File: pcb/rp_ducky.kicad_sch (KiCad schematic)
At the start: 31 parts, among them J1 USB_A, SW1 R-667799, SW2 R-667799, U1 TCR2EE33, U2 W25Q32JVZP, U3 RP2040, Y1 Crystal_GND24

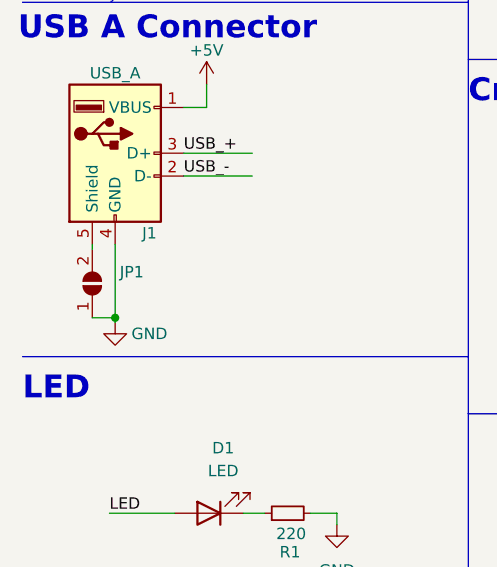
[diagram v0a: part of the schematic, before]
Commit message: WIP
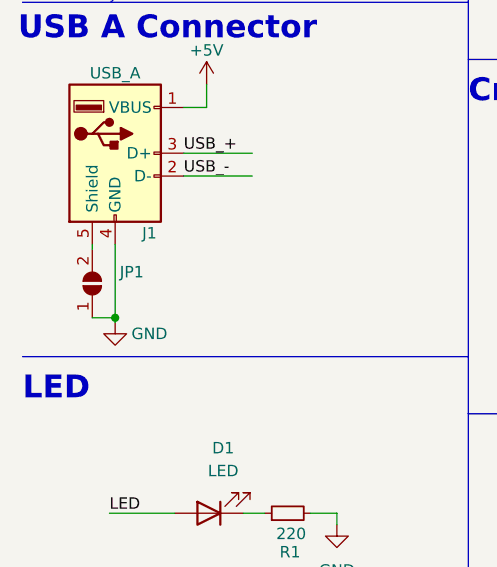
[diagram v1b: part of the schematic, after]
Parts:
- JP1: footprint Jumper:SolderJumper-2_P1.3mm_Open_TrianglePad1.0x1.5mm -> Jumper:SolderJumper-2_P1.3mm_Bridged_RoundedPad1.0x1.5mm
